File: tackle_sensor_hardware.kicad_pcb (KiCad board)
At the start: 4 copper layers, 45.1 x 57.2 mm, 73 parts, among them J1 Conn_01x02_Male, J2 Conn_01x04_Male, J3 Conn_01x03_Male, J4 Conn_ARM_JTAG_SWD_10, Q1 DMP4051LK3, Q9 CSD19538Q3A, SW1 PTS645SL43SMTR92 LFS, SW2 SW_DPDT_x2, T1 DRQ125-330-R, U1 LIS2DE12, U2 STM32G031Fx, U3 LM3488, U4 LD1117S33TR_SOT223, U5 ULN2003ADR

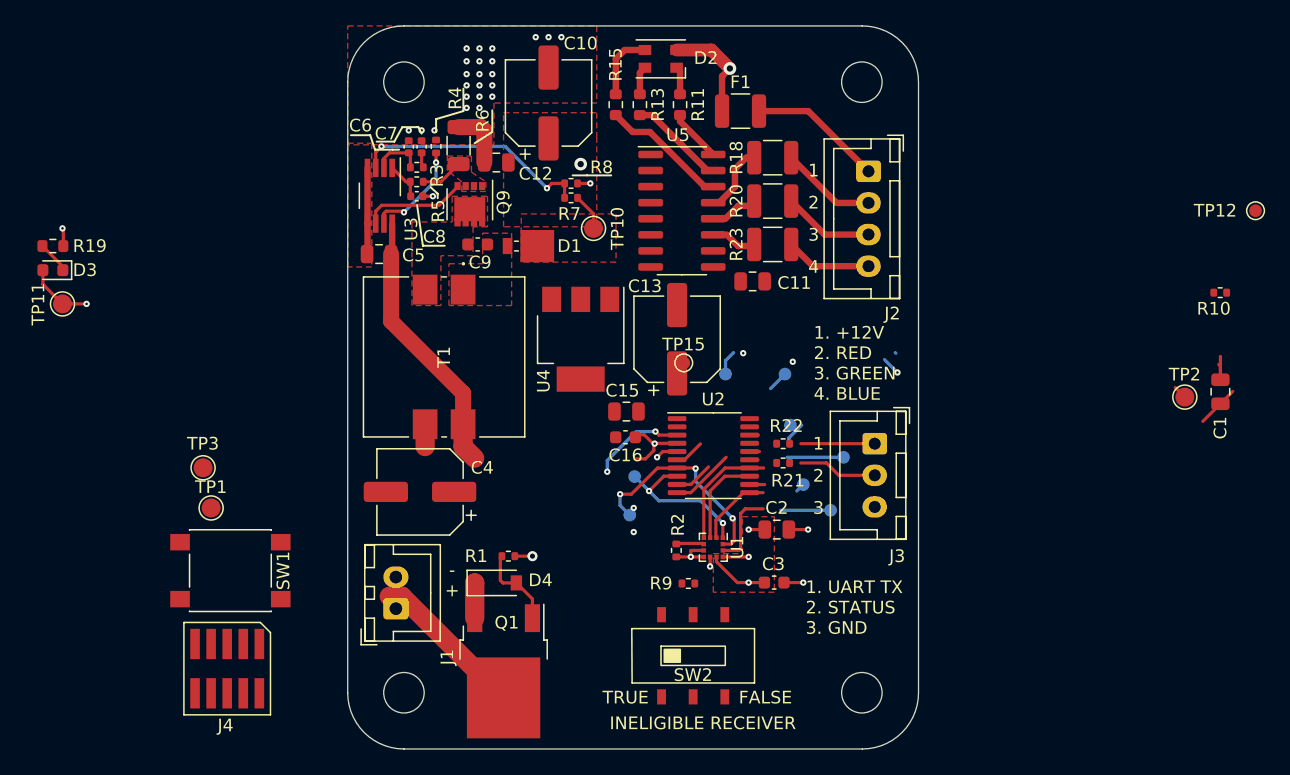
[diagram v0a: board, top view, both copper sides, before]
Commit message: updating the BOM
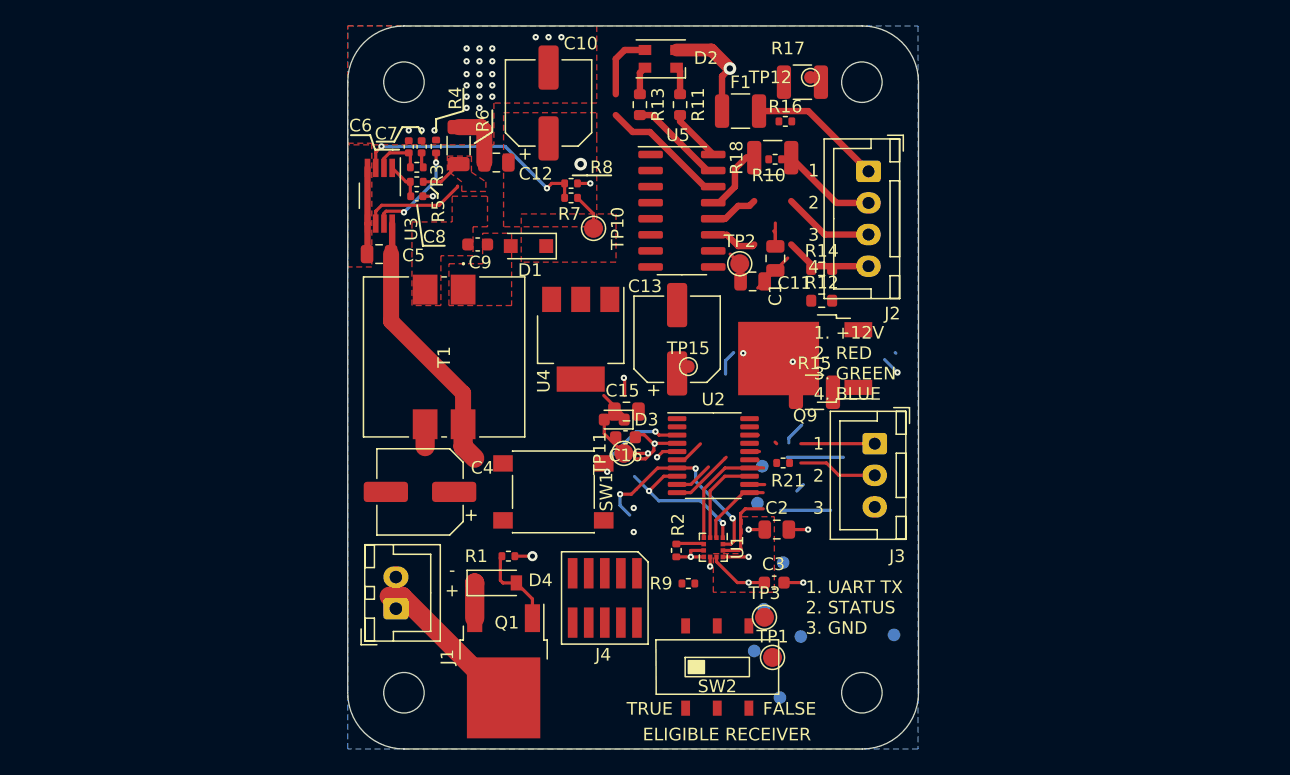
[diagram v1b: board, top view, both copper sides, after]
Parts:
- removed the G*** at (198.6, 81.0)
- removed R19: 1k,1%,25mW, Resistor_SMD:R_0603_1608Metric
- removed R20, R23: 0,0.5W, Resistor_SMD:R_1210_3225Metric
- removed R22: 220,1%,63mW, Resistor_SMD:R_0402_1005Metric
- added G***: LOGO, rfc_footprint_lib:new_logo, B.Cu at (143.4, 95.5)
- added G***: LOGO, rfc_footprint_lib:new_logo_highlights, B.Cu at (143.4, 95.5)
- added R12: 1k,1%,25mW, Resistor_SMD:R_0603_1608Metric, F.Cu at (158.1, 91.6)
- added R14: 1k,1%,25mW, Resistor_SMD:R_0603_1608Metric, F.Cu at (158.1, 89.1)
- added R16: 220,1%,63mW, Resistor_SMD:R_0402_1005Metric, F.Cu at (155.2, 77.4)
- added R17: 0,0.5W, Resistor_SMD:R_1210_3225Metric, F.Cu at (156.6, 74.3)
- D1: value SS2PH10HM3_A/H -> DSK34; footprint Diode_SMD:D_Powermite_AK -> Diode_SMD:D_SOD-123F
- Q9: value CSD19538Q3A -> NCE0110K; footprint Package_SON:VSON-8_3.3x3.3mm_P0.65mm_NexFET -> Package_TO_SOT_SMD:TO-252-2
- R15: value 1k,1%,25mW -> 0,0.5W; footprint Resistor_SMD:R_0603_1608Metric -> Resistor_SMD:R_1210_3225Metric
- moved D3 45.9 mm to (141.7, 101.0)
- moved TP11 45.9 mm to (142.5, 103.6)
- moved TP3 45.9 mm to (153.6, 116.6)
- moved TP1 45.9 mm to (154.2, 119.8)
- moved C1 36.7 mm to (154.5, 88.2)
- moved R10 36.7 mm to (154.4, 80.4)
- moved TP12 36.7 mm to (157.2, 73.9)
- moved TP2 36.7 mm to (151.6, 88.6)
- moved J4 30.4 mm to (141.0, 115.1)
- moved Q9 29.2 mm to (156.8, 96.1), turned to 180 degrees
- moved R15 27.6 mm to (157.5, 98.8), turned to 0 degrees
- moved SW1 26.3 mm to (136.9, 106.7)
- moved TP7 24.0 mm to (163.8, 118.0)
- moved TP8 18.7 mm to (154.8, 122.9)
- moved TP6 14.6 mm to (156.5, 118.1)
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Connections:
- Q9 pad 2: Net-(Q9-Pad1) -> Net-(C9-Pad2)
- Q9 pad 3: Net-(Q9-Pad1) -> Net-(Q9-Pad2)
- R10 pad 1: /SWCLK -> Net-(R7-Pad2)
- R13 pad 1: Net-(D2-Pad4) -> Net-(D2-Pad3)
- R13 pad 2: Net-(R13-Pad2) -> Net-(U5-Pad14)
- R15 pad 1: Net-(D2-Pad3) -> Net-(U5-Pad12)
- R15 pad 2: Net-(R15-Pad2) -> Net-(J2-Pad3)
- R5 pad 2: Net-(Q9-Pad1) -> Net-(Q9-Pad2)
- R6 pad 1: Net-(Q9-Pad1) -> Net-(Q9-Pad2)
- R8 pad 1: Net-(R7-Pad2) -> GND
- R8 pad 2: GND -> /SWCLK
- U3 pad 6: Net-(Q9-Pad4) -> Net-(Q9-Pad1)
- U5 pad 12: Net-(R20-Pad1) -> Net-(U5-Pad12)
- U5 pad 14: Net-(R15-Pad2) -> Net-(U5-Pad14)
- U5 pad 15: Net-(R13-Pad2) -> Net-(U5-Pad15)
- U5 pad 7: unconnected-(U5-Pad7) -> GND
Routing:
- net Net-(U5-Pad14): track 0.00 -> 10.0 mm
- net Net-(R15-Pad2): track 10.0 -> 0.00 mm
- net Net-(Q9-Pad4): track 8.31 -> 0.00 mm
- net Net-(U5-Pad15): track 0.00 -> 7.61 mm
- net Net-(R13-Pad2): track 7.61 -> 0.00 mm
- net Net-(Q9-Pad1): track 3.57 -> 8.31 mm
- net Net-(U5-Pad12): track 0.00 -> 3.82 mm
- net Net-(R20-Pad1): track 3.82 -> 0.00 mm
- net Net-(Q9-Pad2): track 0.00 -> 3.57 mm
- net Net-(D2-Pad4): track 2.26 -> 0.00 mm
- net Net-(D2-Pad3): track 5.39 -> 7.65 mm
- net GND: track 30.3 -> 29.4 mm, vias 33 -> 32
- net /SWCLK: track 0.59 -> 1.48 mm
- net Net-(C9-Pad2): vias 0 -> 2
- net /RST: vias 1 -> 0
- added copper zone on B.Cu, net GND
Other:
- board text added: "ELIGIBLE RECEIVER"
- board text removed: "INELIGIBLE RECEIVER"
